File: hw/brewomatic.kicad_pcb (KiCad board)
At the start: 2 copper layers, 95.2 x 78.7 mm, 29 parts, among them J1 CON_MAX31865, J2 EXP1, J3 EXP2, J4 12V_IN, J5 230V_CONN, J6 HEATING_CONN, J7 PUMP_CONN, J8 12V_ALIM_CONN, Q1 BT139-600, Q2 IRF540N, U1 MOC3021M, U2 4N25, U3 4N25

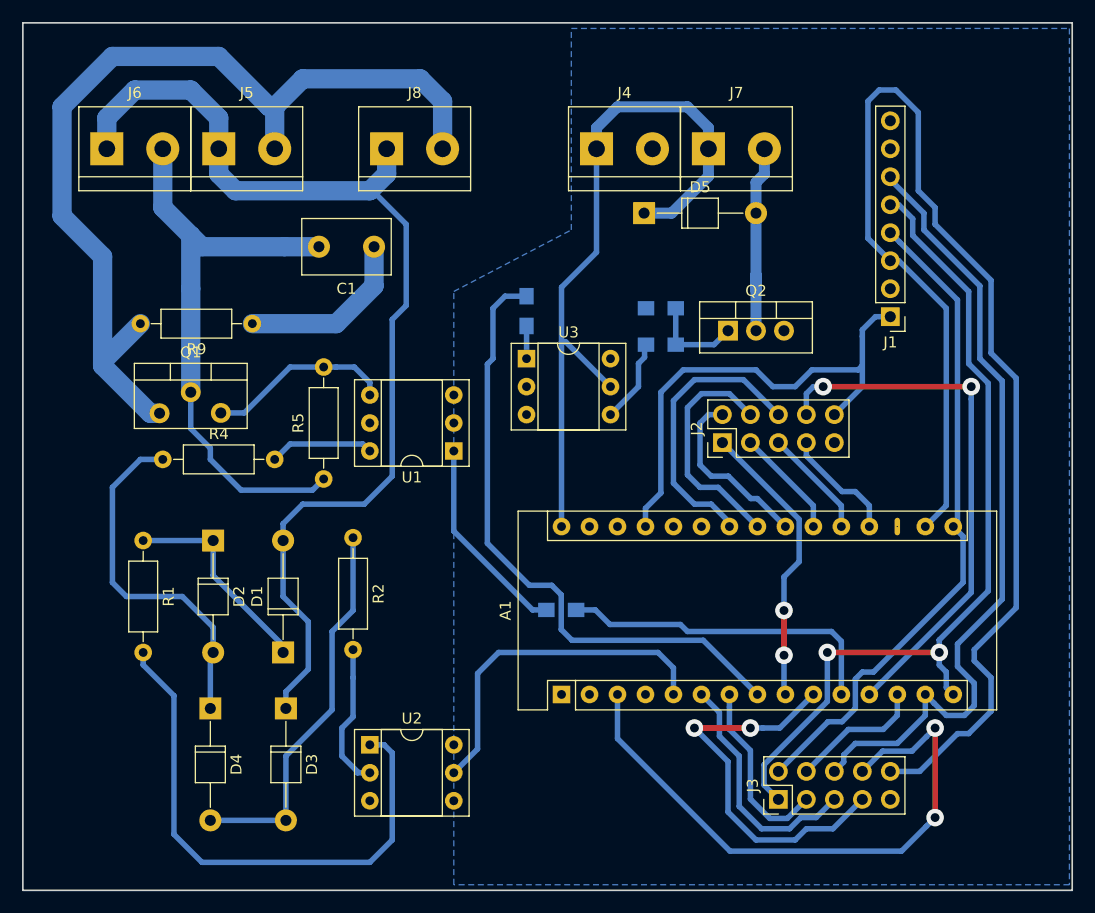
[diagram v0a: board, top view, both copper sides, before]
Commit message: PCB: finalize layout
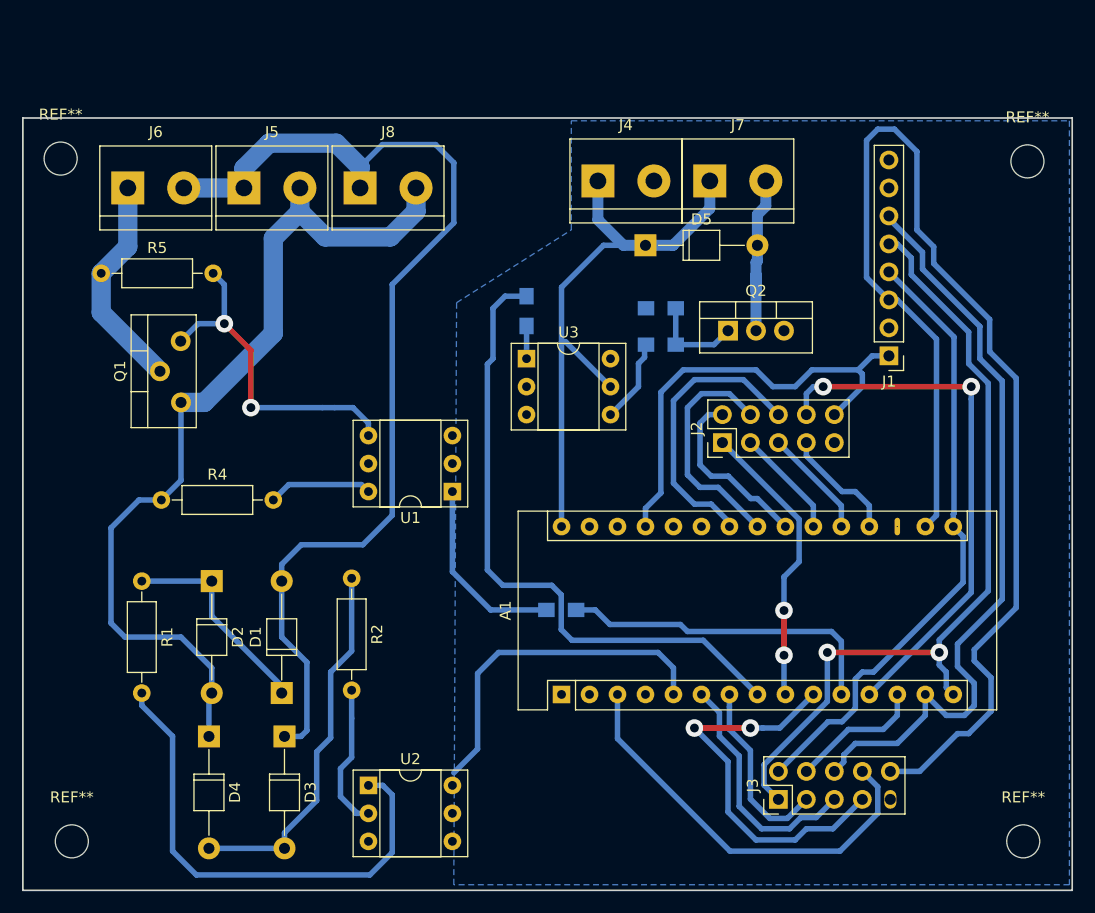
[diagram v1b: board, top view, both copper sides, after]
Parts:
- removed C1: C, Capacitors_THT:C_Disc_D8.0mm_W5.0mm_P5.00mm
- removed R9: R, Resistors_THT:R_Axial_DIN0207_L6.3mm_D2.5mm_P10.16mm_Horizontal
- added REF**: MountingHole_3mm, Mounting_Holes:MountingHole_3mm, F.Cu at (120.3, 91.1)
- added REF**: MountingHole_3mm, Mounting_Holes:MountingHole_3mm, F.Cu at (208.0, 91.3)
- added REF**: MountingHole_3mm, Mounting_Holes:MountingHole_3mm, F.Cu at (121.3, 153.0)
- added REF**: MountingHole_3mm, Mounting_Holes:MountingHole_3mm, F.Cu at (207.6, 153.0)
- R1: value R -> 45K
- R2: value R -> R45K
- moved R5 27.5 mm to (124.0, 101.5), turned to 0 degrees
- moved J8 4.30 mm to (147.4, 93.7)
- moved J5 4.23 mm to (136.9, 93.7)
- moved J6 4.03 mm to (126.4, 93.7)
- moved U2 3.69 mm to (148.2, 148.0)
- moved D1 3.69 mm to (140.3, 139.6)
- moved D2 3.69 mm to (134.0, 129.4)
- moved R1 3.69 mm to (127.6, 129.4)
- moved R2 3.69 mm to (146.7, 129.2)
- moved R4 3.69 mm to (129.4, 122.0)
- moved U1 3.69 mm to (155.8, 121.3)
- moved J1 3.56 mm to (195.5, 109.0)
- moved D5 2.92 mm to (173.4, 98.9)
- moved J4 2.92 mm to (169.0, 93.1)
- moved J7 2.92 mm to (179.2, 93.1)
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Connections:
- J6 pad 1: NEUT -> /HEATING_LINE
- J6 pad 2: /HEATING_LINE -> NEUT
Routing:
- net LINE: track 118.1 -> 80.8 mm
- net /HEATING_LINE: track 53.9 -> 19.8 mm
- net /RST: track 54.7 -> 37.7 mm, vias 2 -> 0
- net Net-(C1-Pad1): track 16.0 -> 0.00 mm
- net Net-(Q1-Pad3): track 17.0 -> 30.6 mm, vias 0 -> 2
- net +12V: track 67.0 -> 55.6 mm
- net +3V3: track 120.3 -> 112.5 mm
- net Net-(R1-Pad2): track 49.6 -> 44.9 mm
- net +5V: track 45.1 -> 41.4 mm
- net /SPI_MOSI: track 72.8 -> 69.3 mm
- net /SPI_MISO: track 77.4 -> 73.9 mm
- net /SPI_SCK: track 60.2 -> 57.0 mm
- net Net-(D5-Pad2): track 18.3 -> 15.5 mm
- net /PUMP_CTRL: track 57.1 -> 58.5 mm
- net Net-(R3-Pad1): track 18.6 -> 17.2 mm
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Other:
- board size 95.2 x 78.7 mm -> 95.2 x 70.1 mm
